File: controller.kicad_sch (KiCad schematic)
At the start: 40 parts, among them U3 STM32F767ZITx, Y1 25MHz

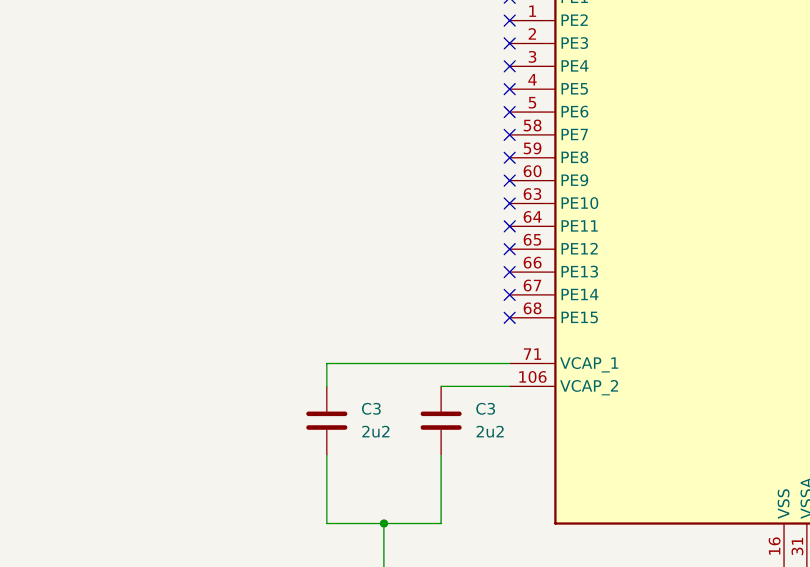
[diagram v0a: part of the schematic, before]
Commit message: Board outline finished, component placement, added markers, added annotations, etc.
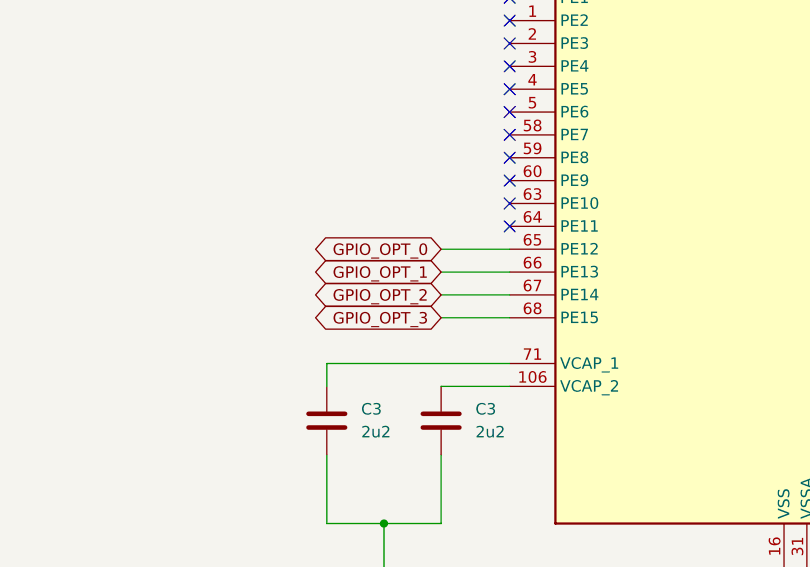
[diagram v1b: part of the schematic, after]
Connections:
- net GPIO_OPT_0: now reaches U3.65 (PE12)
- net GPIO_OPT_1: now reaches U3.66 (PE13)
- net GPIO_OPT_2: now reaches U3.67 (PE14)
- net GPIO_OPT_3: now reaches U3.68 (PE15)
- no-connect marks 87 -> 83
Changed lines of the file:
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@@
   )
   (no_connect (at 185.42 157.48))
-  (no_connect (at 185.42 210.82))
   (no_connect (at 185.42 167.64))
   (no_connect (at 246.38 218.44))
@@
   (no_connect (at 246.38 127))
   (no_connect (at 185.42 170.18))
-  (no_connect (at 185.42 218.44))
   (no_connect (at 246.38 205.74))
   (no_connect (at 185.42 195.58))
@@
   (no_connect (at 246.38 180.34))
   (no_connect (at 246.38 165.1))
-  (no_connect (at 185.42 215.9))
   (no_connect (at 185.42 193.04))
   (no_connect (at 246.38 220.98))
@@
   (no_connect (at 246.38 124.46))
   (no_connect (at 246.38 200.66))
-  (no_connect (at 185.42 213.36))
   (no_connect (at 185.42 185.42))
   (no_connect (at 246.38 132.08))
@@
     (stroke (width 0) (type default))
   )
+  (wire (pts (xy 177.8 215.9) (xy 185.42 215.9))
+    (stroke (width 0) (type default))
+  )
   (wire (pts (xy 246.38 144.78) (xy 254 144.78))
     (stroke (width 0) (type default))
@@
     (stroke (width 0) (type default))
   )
+  (wire (pts (xy 177.8 210.82) (xy 185.42 210.82))
+    (stroke (width 0) (type default))
+  )
   (wire (pts (xy 246.38 160.02) (xy 254 160.02))
     (stroke (width 0) (type default))
@@
     (stroke (width 0) (type default))
   )
+  (wire (pts (xy 177.8 213.36) (xy 185.42 213.36))
+    (stroke (width 0) (type default))
+  )
   (wire (pts (xy 233.68 55.88) (xy 233.68 60.96))
     (stroke (width 0) (type default))
@@
   )
   (wire (pts (xy 205.74 58.42) (xy 205.74 60.96))
+    (stroke (width 0) (type default))
+  )
+  (wire (pts (xy 177.8 218.44) (xy 185.42 218.44))
     (stroke (width 0) (type default))
   )
@@
     )
   )
+  (global_label "GPIO_OPT_2" (shape bidirectional) (at 177.8 215.9 180) (fields_autoplaced)
+    (effects (font (size 1.27 1.27)) (justify right))
+    (property "Intersheetrefs" "${INTERSHEET_REFS}" (at 162.5154 215.9 0)
+      (effects (font (size 1.27 1.27)) (justify right) hide)
+    )
+  )
+  (global_label "GPIO_OPT_3" (shape bidirectional) (at 177.8 218.44 180) (fields_autoplaced)
+    (effects (font (size 1.27 1.27)) (justify right))
+    (property "Intersheetrefs" "${INTERSHEET_REFS}" (at 162.5154 218.44 0)
+      (effects (font (size 1.27 1.27)) (justify right) hide)
+    )
+  )
   (global_label "GEN_REFCLK" (shape output) (at 254 170.18 0) (fields_autoplaced)
     (effects (font (size 1.27 1.27)) (justify left))
@@
     )
   )
+  (global_label "GPIO_OPT_0" (shape bidirectional) (at 177.8 210.82 180) (fields_autoplaced)
+    (effects (font (size 1.27 1.27)) (justify right))
+    (property "Intersheetrefs" "${INTERSHEET_REFS}" (at 162.5154 210.82 0)
+      (effects (font (size 1.27 1.27)) (justify right) hide)
+    )
+  )
   (global_label "MCU_CRYSTAL_PH0" (shape passive) (at 175.26 86.36 180) (fields_autoplaced)
     (effects (font (size 1.27 1.27)) (justify right))
@@
     )
   )
+  (global_label "GPIO_OPT_1" (shape bidirectional) (at 177.8 213.36 180) (fields_autoplaced)
+    (effects (font (size 1.27 1.27)) (justify right))
+    (property "Intersheetrefs" "${INTERSHEET_REFS}" (at 162.5154 213.36 0)
+      (effects (font (size 1.27 1.27)) (justify right) hide)
+    )
+  )
